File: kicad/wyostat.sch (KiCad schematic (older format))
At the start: 71 parts, among them J1 PWR_In, J10 MOSI, J11 RST, J12 GND, J13 AC_IN, J14 ~RST, J2 OUT1, J3 OUT2, J4 I2C_ext1, J5 MISO, J6 3V3, J7 OUT3, J8 SCK, J9 SPI, Q1 BT136-600, Q2 BT136-600, Q3 BT136-600, U1 MOC3063M, U2 Wemos-Lolin, U3 MOC3063M, U4 MOC3063M, U5 MAX17502FATB+T

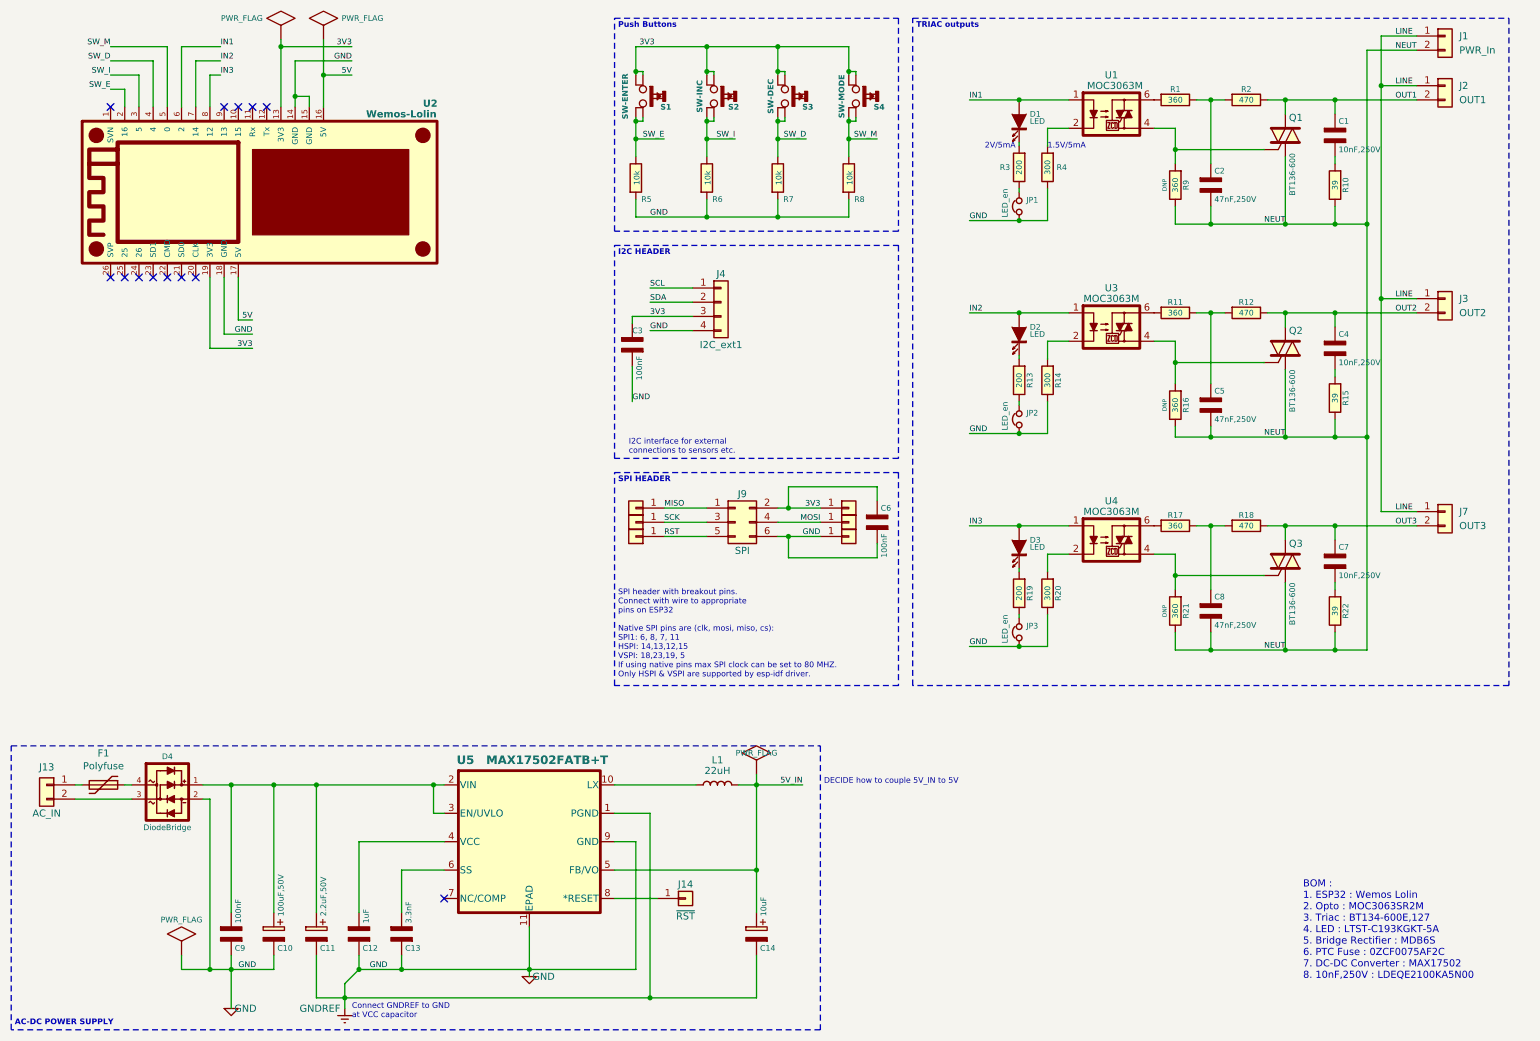
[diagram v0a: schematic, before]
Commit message: kicad schematic, WIP
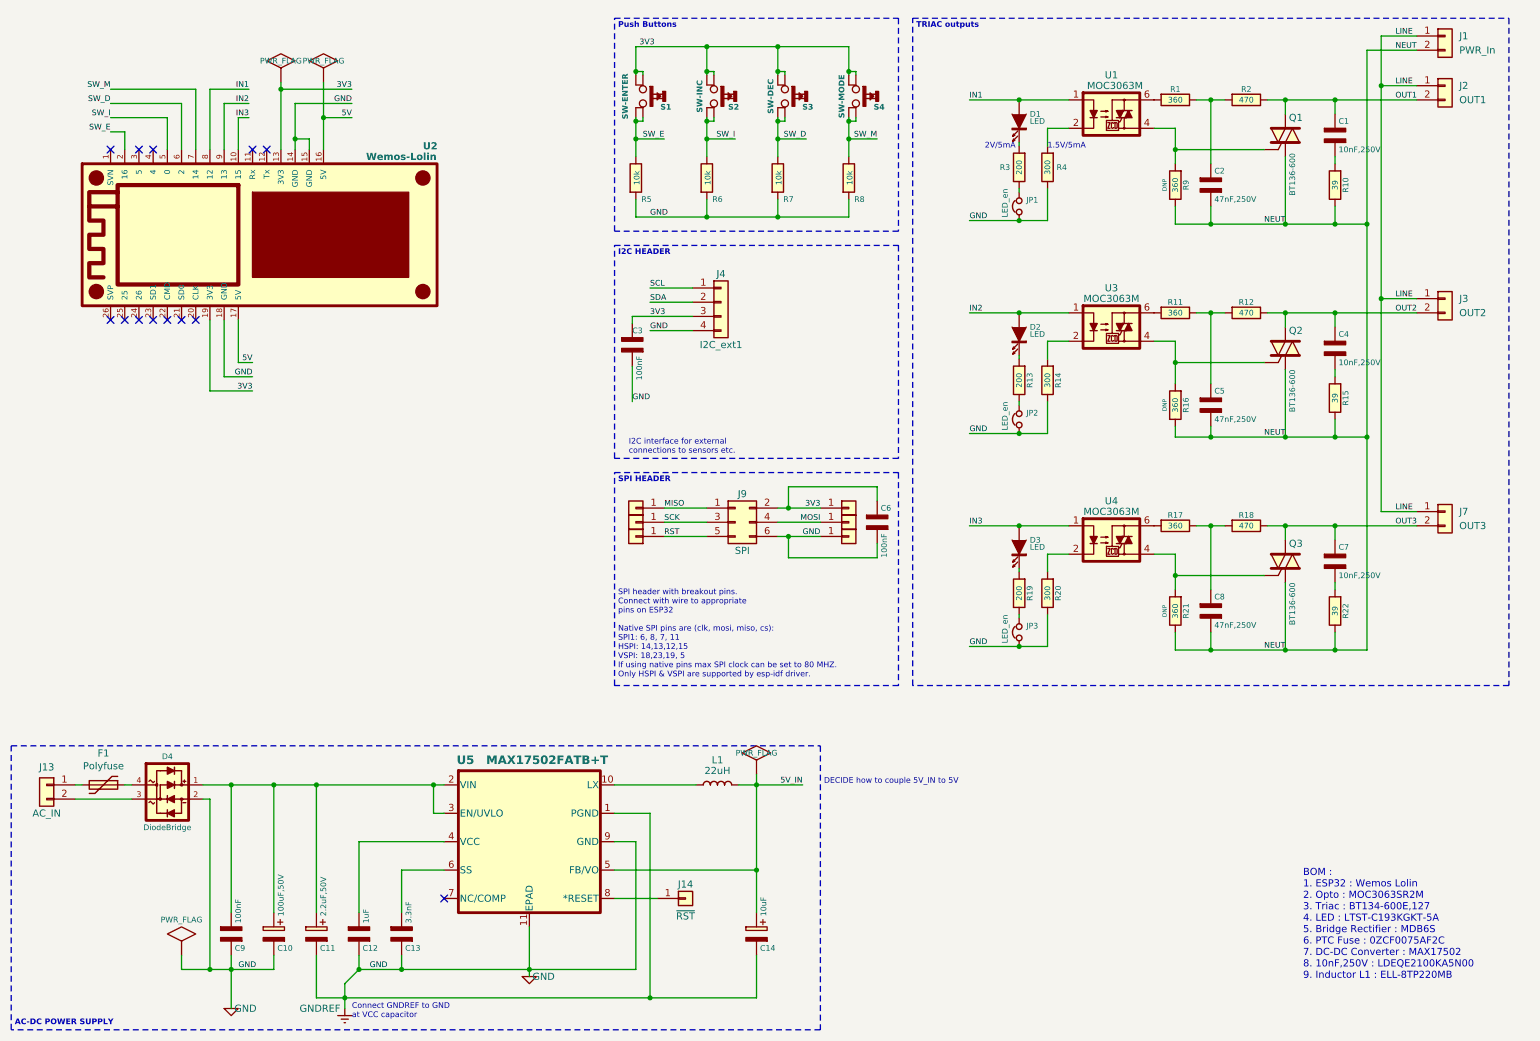
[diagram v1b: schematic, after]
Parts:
- C1: footprint Capacitors_Tantalum_SMD:CP_Tantalum_Case-E_EIA-7260-38_Hand -> wyostat_fp:C_2220
- C10, C2, C4, C5, C7, C8: footprint (none) -> wyostat_fp:C_2220
- C11, C12, C13, C14, C3, C6, C9: footprint Capacitors_SMD:C_0805 -> wyostat_fp:C_0805
- D1, D2, D3: footprint LEDs:LED_0603 -> wyostat_fp:LED_0603
- D4: footprint (none) -> wyostat_fp:Diode_bridge
- F1: footprint Fuse_Holders_and_Fuses:Fuse_SMD2920 -> wyostat_fp:Fuse_SMD2920
- J1, J13, J2, J3, J7: footprint Connectors_Terminal_Blocks:TerminalBlock_Pheonix_MPT-2.54mm_2pol -> wyostat_fp:TerminalBlock_Pheonix_MPT-2.54mm_2pol
- J10, J11, J12, J14, J5, J6, J8: footprint Pin_Headers:Pin_Header_Straight_1x01 -> wyostat_fp:Pin_Header_Straight_1x01
- J4: footprint Pin_Headers:Pin_Header_Straight_1x04 -> wyostat_fp:Pin_Header_Straight_1x04
- J9: footprint Pin_Headers:Pin_Header_Straight_2x03 -> wyostat_fp:Pin_Header_Straight_2x03
- JP1, JP2, JP3: footprint LEDs:LED_0402 -> wyostat_fp:LED_0402
- L1: footprint (none) -> wyostat_fp:Inductor_ELL8TP
- Q1, Q2, Q3: footprint TO_SOT_Packages_THT:TO-220_Neutral123_Vertical -> wyostat_fp:SOT126_SOT32_Housing_Horizontal
- R1, R10, R11, R12, R13, R14, R15, R16, R17, R18, R19, R2, R20, R21, R22, R3, R4, R5, R6, R7, R8, R9: footprint Resistors_SMD:R_0805 -> wyostat_fp:R_0805
- S1, S2, S3, S4: footprint KlokTHREEjr_libs:SW_SMD -> wyostat_fp:SW_SPST_CK_KSCx
- U1, U3, U4: footprint Opto-Devices:Optocoupler_6pin_wide_Stile-I -> wyostat_fp:Optocoupler_6pin
- U2: footprint (none) -> wyostat_fp:Wemos_Lolin
- U5: footprint (none) -> wyostat_fp:TDFN-10
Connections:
- net IN1: now also U2.8 (12); no longer U2.6 (2)
- net IN2: now also U2.9 (13); no longer U2.7 (14)
- net IN3: now also U2.10 (15); no longer U2.8 (12)
- net SW_D: now also U2.6 (2); no longer U2.4
- net SW_I: now also U2.5 (0); no longer U2.3 (5)
- net SW_M: now also U2.7 (14); no longer U2.5 (0)
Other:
- note added: "BOM :\n1. ESP32 : Wemos Lolin\n2. Opto : MOC3063SR2M\n3. Triac : BT134-600E,127\n4. LED : LTST-C193KGKT-5A\n5. Bridge Rectifier : MDB6S\n6. PTC Fuse : 0ZCF0075AF2C\n7. DC-DC Converter : MAX17502\n8. 10nF,250V : LDEQE2100KA5N00\n9. Inductor L1 : ELL-8TP220MB"
- note removed: "BOM :\n1. ESP32 : Wemos Lolin\n2. Opto : MOC3063SR2M\n3. Triac : BT134-600E,127\n4. LED : LTST-C193KGKT-5A\n5. Bridge Rectifier : MDB6S\n6. PTC Fuse : 0ZCF0075AF2C\n7. DC-DC Converter : MAX17502\n8. 10nF,250V : LDEQE2100KA5N00"
- moved on the sheet: U2

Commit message: kicad schematic, WIP
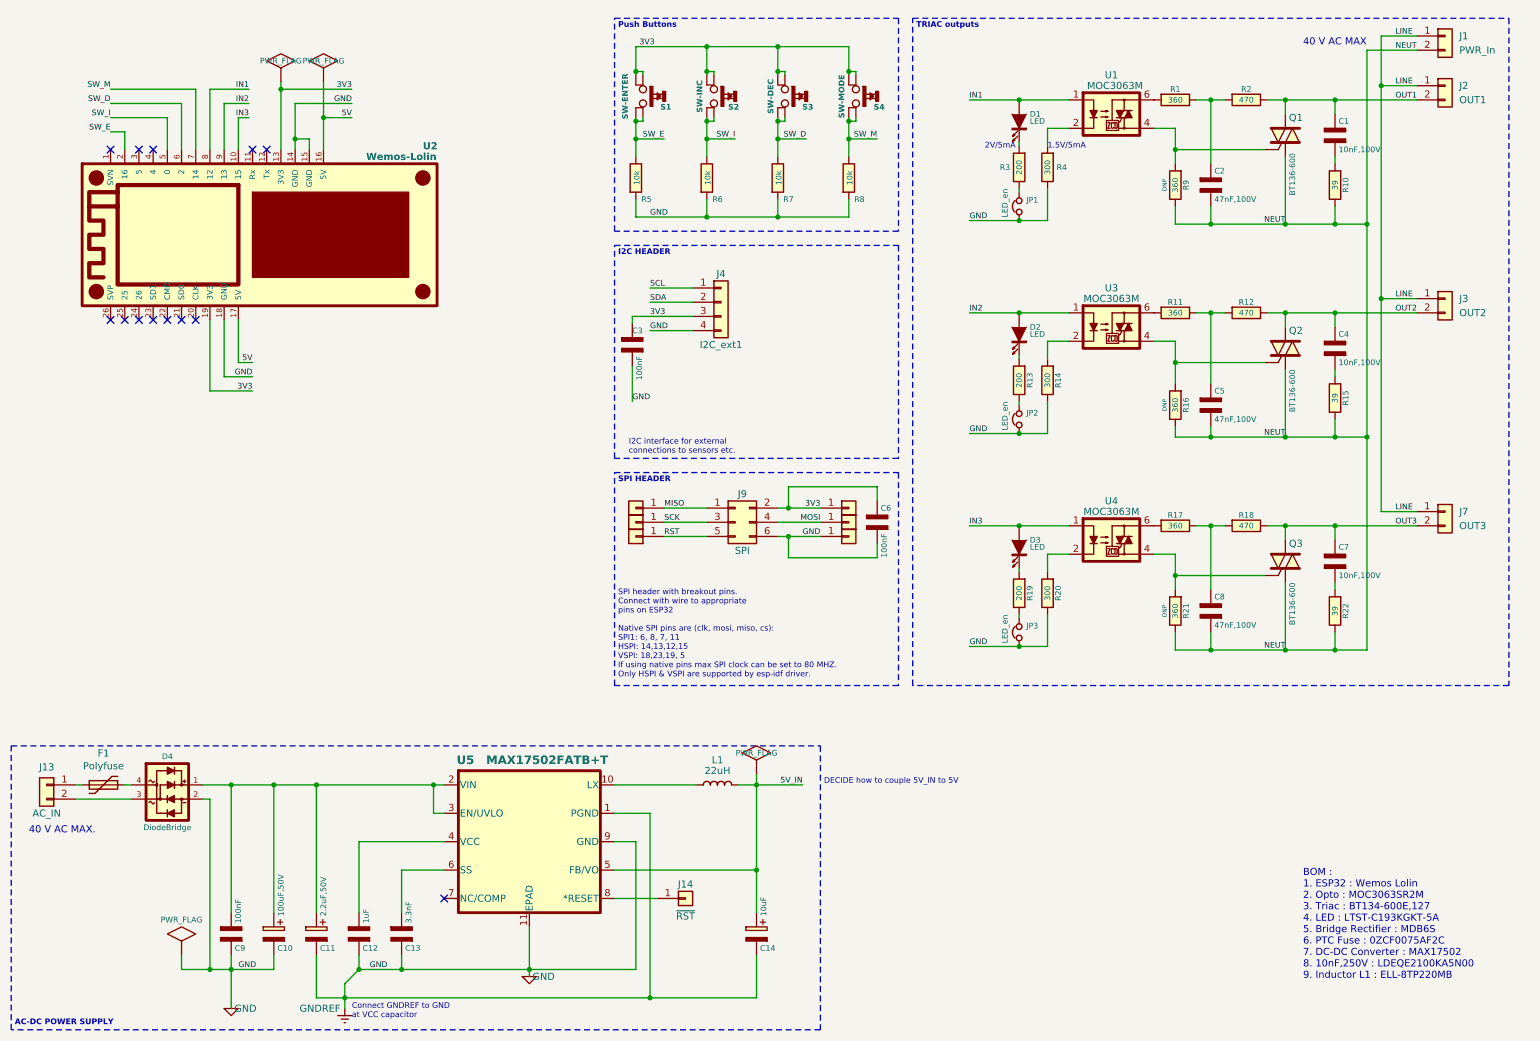
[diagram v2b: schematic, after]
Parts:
- C1, C4, C7: value 10nF,250V -> 10nF,100V
- C2, C5, C8: value 47nF,250V -> 47nF,100V
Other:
- note added: "40 V AC MAX"
- note added: "40 V AC MAX."
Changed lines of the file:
@@
 P 9025 1750
 F 0 "C2" H 9050 1850 40  0000 L CNN
-F 1 "47nF,250V" H 9050 1650 40  0000 L CNN
+F 1 "47nF,100V" H 9050 1650 40  0000 L CNN
 F 2 "wyostat_fp:C_2220" H 9025 1750 60  0001 C CNN
 F 3 "" H 9025 1750 60  0000 C CNN
@@
 P 9025 3300
 F 0 "C5" H 9050 3400 40  0000 L CNN
-F 1 "47nF,250V" H 9050 3200 40  0000 L CNN
+F 1 "47nF,100V" H 9050 3200 40  0000 L CNN
 F 2 "wyostat_fp:C_2220" H 9025 3300 60  0001 C CNN
 F 3 "" H 9025 3300 60  0000 C CNN
@@
 P 9025 4750
 F 0 "C8" H 9050 4850 40  0000 L CNN
-F 1 "47nF,250V" H 9050 4650 40  0000 L CNN
+F 1 "47nF,100V" H 9050 4650 40  0000 L CNN
 F 2 "wyostat_fp:C_2220" H 9025 4750 60  0001 C CNN
 F 3 "" H 9025 4750 60  0000 C CNN
@@
 P 9900 1400
 F 0 "C1" H 9925 1500 40  0000 L CNN
-F 1 "10nF,250V" H 9925 1300 40  0000 L CNN
+F 1 "10nF,100V" H 9925 1300 40  0000 L CNN
 F 2 "wyostat_fp:C_2220" H 9900 1400 60  0001 C CNN
 F 3 "" H 9900 1400 60  0000 C CNN
@@
 P 9900 2900
 F 0 "C4" H 9925 3000 40  0000 L CNN
-F 1 "10nF,250V" H 9925 2800 40  0000 L CNN
+F 1 "10nF,100V" H 9925 2800 40  0000 L CNN
 F 2 "wyostat_fp:C_2220" H 9900 2900 60  0001 C CNN
 F 3 "" H 9900 2900 60  0000 C CNN
@@
 P 9900 4400
 F 0 "C7" H 9925 4500 40  0000 L CNN
-F 1 "10nF,250V" H 9925 4300 40  0000 L CNN
+F 1 "10nF,100V" H 9925 4300 40  0000 L CNN
 F 2 "wyostat_fp:C_2220" H 9900 4400 60  0001 C CNN
 F 3 "" H 9900 4400 60  0000 C CNN
@@
 EndData
 $EndBitmap
+Text Notes 700  6325 0    50   ~ 0
+40 V AC MAX.
+Text Notes 9675 775  0    50   ~ 0
+40 V AC MAX
 $EndSCHEMATC

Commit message: schematic WIP
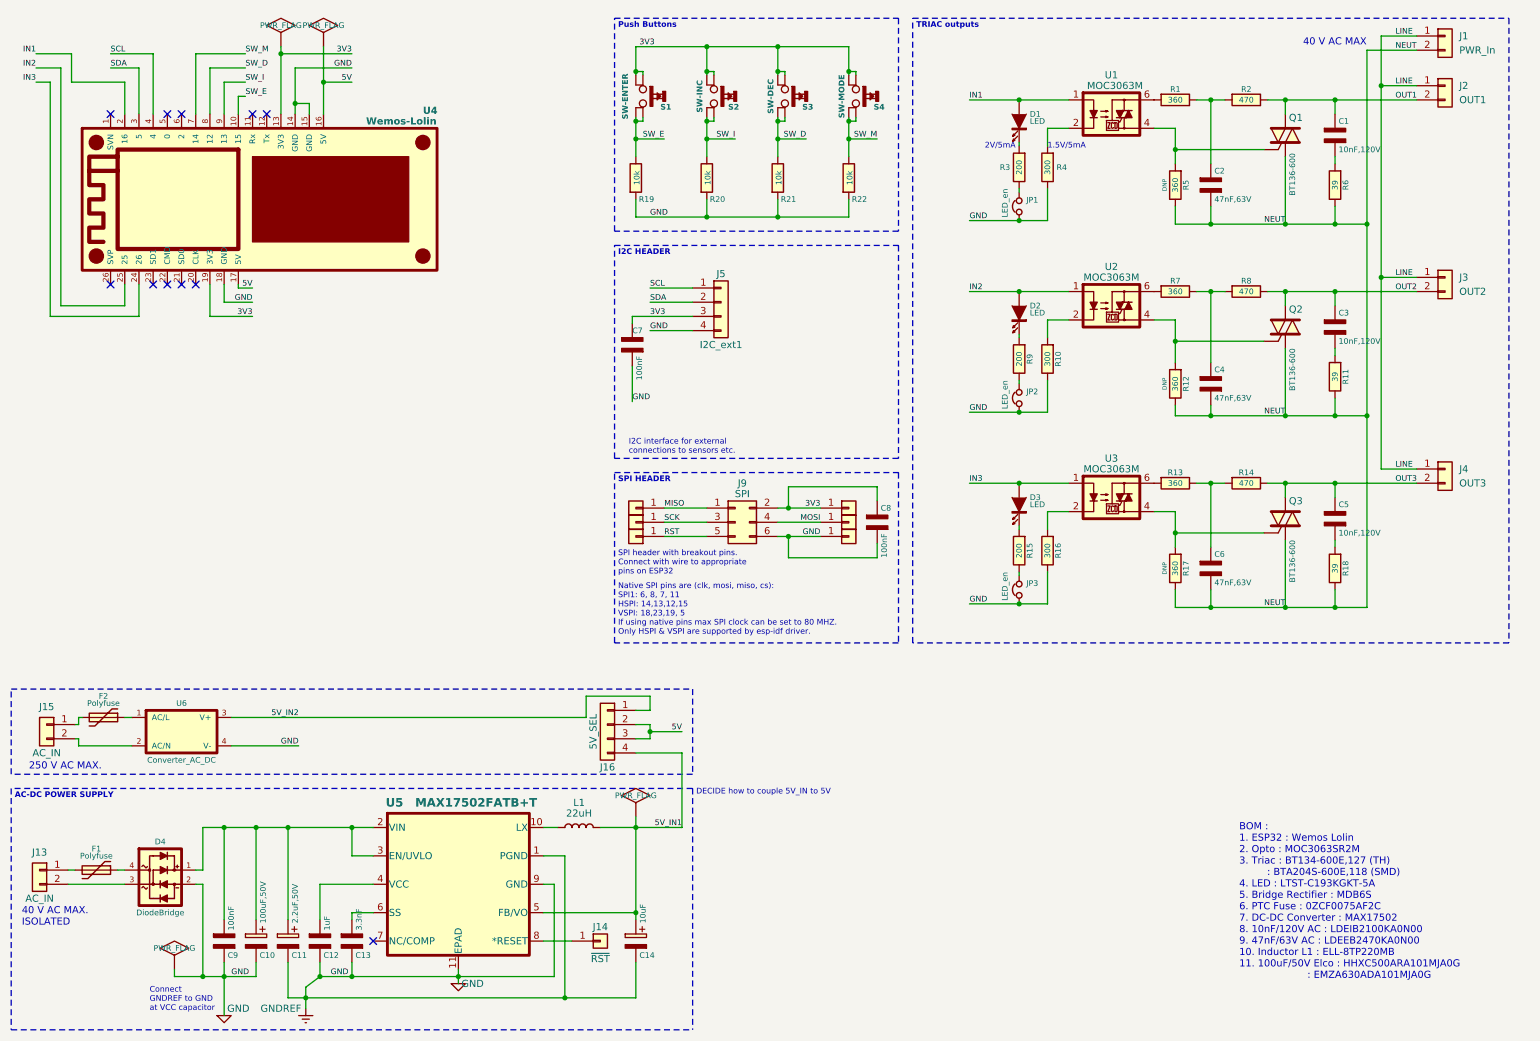
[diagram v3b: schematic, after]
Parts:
- added F2: Polyfuse, wyostat_fp:Fuse_SMD2920, symbol wyostat:Polyfuse
- added J15: AC_IN, wyostat_fp:TerminalBlock_Pheonix_MPT-2.54mm_2pol, symbol wyostat:Conn_01x02
- added J16: 5V_SEL, symbol wyostat:Conn_01x04
- added U6: Converter_AC_DC, symbol wyostat:Converter_AC_DC
- C1: value 10nF,100V -> 10nF,120V
- C10: footprint wyostat_fp:C_2220 -> Capacitors_SMD:CP_Elec_10x10
- C2: value 47nF,100V -> 47nF,63V
- C3: renamed from C4; value 10nF,100V -> 10nF,120V
- C4: renamed from C5; value 47nF,100V -> 47nF,63V
- C5: renamed from C7; value 10nF,100V -> 10nF,120V
- C6: renamed from C8; value 47nF,100V -> 47nF,63V
- Q1, Q2, Q3: footprint wyostat_fp:SOT126_SOT32_Housing_Horizontal -> SMD_Packages:DPAK-2
- renumbered C3 to C7, C6 to C8, J7 to J4, J4 to J5, J5 to J6, J6 to J7, R14 to R10, R15 to R11, R16 to R12, R17 to R13, R18 to R14, R19 to R15, R20 to R16, R21 to R17, R22 to R18, R5 to R19, R6 to R20, R7 to R21, R8 to R22, R9 to R5, R10 to R6, R11 to R7, R12 to R8, R13 to R9, U3 to U2, U4 to U3, U2 to U4
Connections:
- net 5V: now also J16.2 (Pin_2), J16.3 (Pin_3)
- net GND: now also U6.4 (V-)
- net IN1: now also U4.2 (16); no longer U4.8 (12)
- net IN2: now also U4.25; no longer U4.9 (13)
- net IN3: now also U4.24 (26); no longer U4.10 (15)
- net SCL: now also U4.4
- net SDA: now also U4.3 (5)
- net SW_D: now also U4.8 (12); no longer U4.6 (2)
- net SW_E: now also U4.10 (15); no longer U4.2 (16)
- net SW_I: now also U4.9 (13); no longer U4.5 (0)
- net 5V_IN renamed 5V_IN1
- net 5V_IN1: now also J16.4 (Pin_4)
- new net: F2.1, U6.1 (AC/L)
- new net: J15.2 (Pin_2), U6.2 (AC/N)
- new net: F2.2, J15.1 (Pin_1)
- new net 5V_IN2: J16.1 (Pin_1), U6.3 (V+)
- no-connect marks 13 -> 11
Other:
- note added: "250 V AC MAX."
- note added: "40 V AC MAX.\nISOLATED"
- note added: "BOM :\n1. ESP32 : Wemos Lolin\n2. Opto : MOC3063SR2M\n3. Triac : BT134-600E,127 (TH)\n : BTA204S-600E,118 (SMD)\n4. LED : LTST-C193KGKT-5A\n5. Bridge Rectifier : MDB6S\n6. PTC Fuse : 0ZCF0075AF2C\n7. DC-DC Converter : MAX17502\n8. 10nF/120V AC : LDEIB2100KA0N00\n9. 47nF/63V AC : LDEEB2470KA0N00\n10. Inductor L1 : ELL-8TP220MB\n11. 100uF/50V Elco : HHXC500ARA101MJA0G\n : EMZA630ADA101MJA0G"
- note added: "Connect\nGNDREF to GND\nat VCC capacitor"
- note removed: "40 V AC MAX."
- note removed: "BOM :\n1. ESP32 : Wemos Lolin\n2. Opto : MOC3063SR2M\n3. Triac : BT134-600E,127\n4. LED : LTST-C193KGKT-5A\n5. Bridge Rectifier : MDB6S\n6. PTC Fuse : 0ZCF0075AF2C\n7. DC-DC Converter : MAX17502\n8. 10nF,250V : LDEQE2100KA5N00\n9. Inductor L1 : ELL-8TP220MB"
- note removed: "Connect GNDREF to GND\nat VCC capacitor"
- moved on the sheet: C10, C11, C12, C13, C14, C3, C4, C5, C6, C9, D2, D3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
